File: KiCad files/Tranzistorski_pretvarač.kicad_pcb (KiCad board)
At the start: 2 copper layers, 99.9 x 92.6 mm, 30 parts, among them J1 Screw_Terminal_01x01, J2 Screw_Terminal_01x01, J3 Conn_01x03_Male, J4 Conn_01x01_Male, J5 Screw_Terminal_01x01, J6 Conn_01x01_Male, J7 Conn_01x01_Male, J8 Conn_01x01_Male, J9 Screw_Terminal_01x01, Q1 IRLZ44N, U1 SG3524

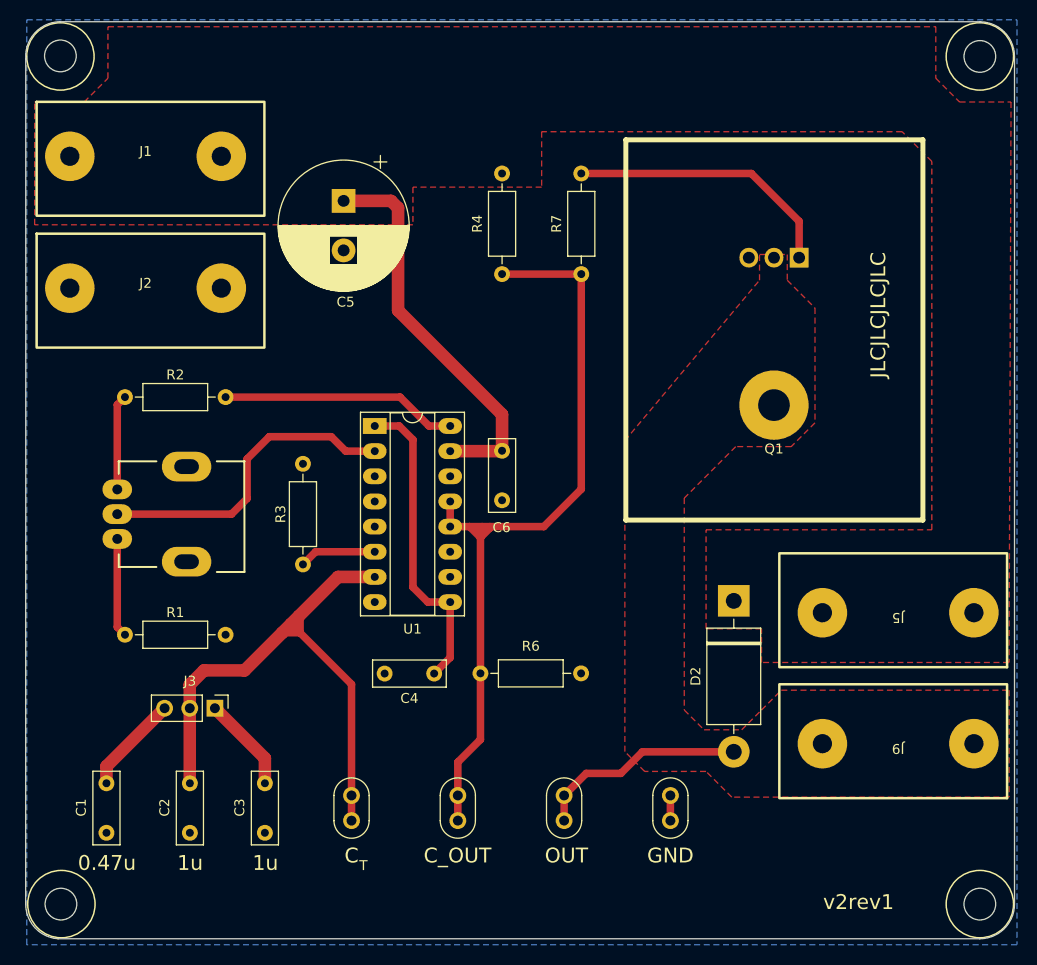
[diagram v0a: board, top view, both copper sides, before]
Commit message: v3
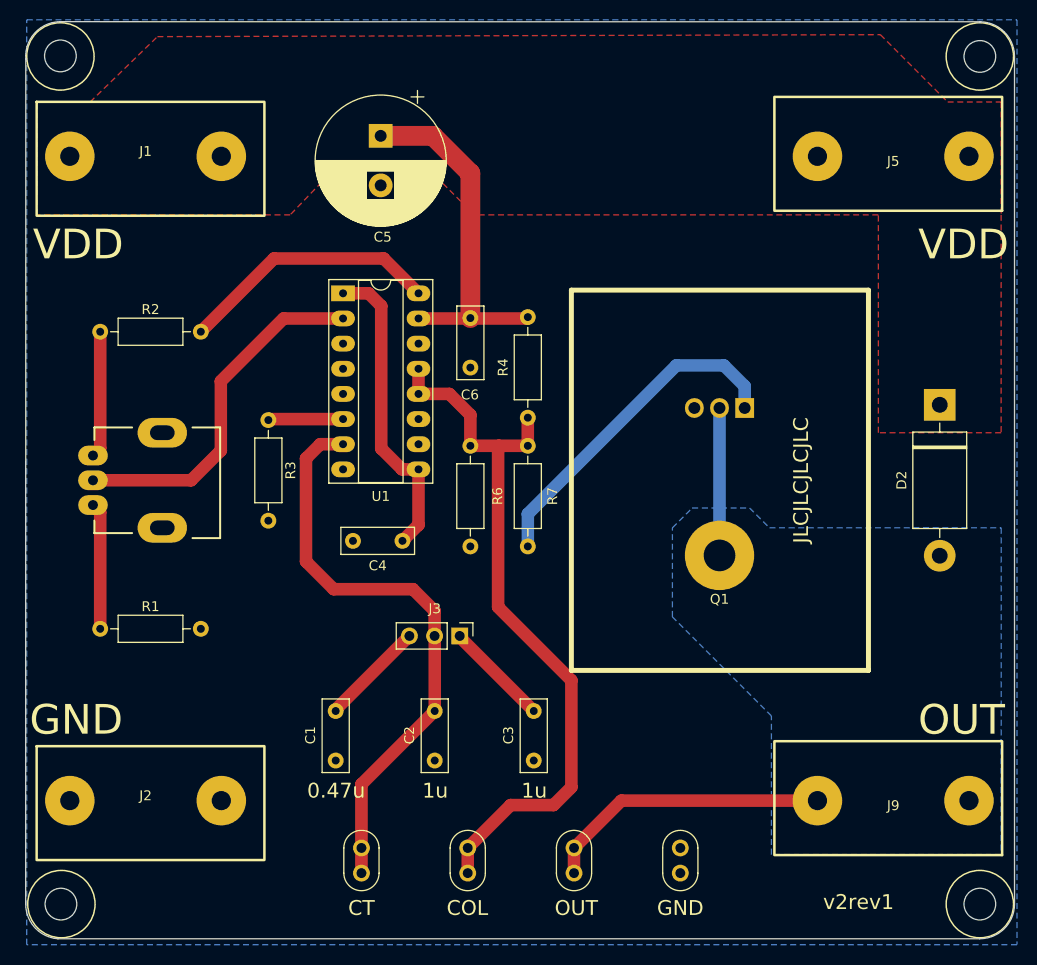
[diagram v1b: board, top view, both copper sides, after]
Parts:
- moved J2 51.8 mm to (101.0, 134.8)
- moved J5 46.1 mm to (176.5, 69.7)
- moved R7 38.0 mm to (139.6, 109.1), turned to 90 degrees
- moved D2 28.7 mm to (181.2, 94.8)
- moved C3 28.1 mm to (140.2, 125.7)
- moved C2 25.8 mm to (130.2, 125.7)
- moved J3 25.8 mm to (132.7, 118.1)
- moved C1 24.3 mm to (120.2, 125.7)
- moved R6 23.0 mm to (133.8, 98.9), turned to -90 degrees
- moved Q1 16.1 mm to (161.5, 95.1)
- moved R3 15.0 mm to (113.4, 96.3), turned to -90 degrees
- moved R4 14.7 mm to (139.6, 85.9)
- moved C4 13.8 mm to (126.9, 108.5)
- moved U1 13.8 mm to (120.9, 83.5)
- moved C6 13.8 mm to (133.8, 86.0)
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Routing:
- net Net-(D2-Pad2): track 21.5 -> 44.0 mm
- net Net-(J6-Pad1): track 80.8 -> 73.5 mm
- net Net-(Q1-Pad1): track 27.7 -> 34.5 mm
- net Net-(RV1-Pad2): track 32.2 -> 36.1 mm
- net VDD: track 39.9 -> 36.3 mm
- net Net-(R2-Pad2): track 9.64 -> 12.8 mm
- net Net-(R1-Pad1): track 10.0 -> 12.8 mm
- net /+5V_REF: track 23.9 -> 26.5 mm
- net GND: track 2.54 -> 0.00 mm
- net Net-(C3-Pad1): track 9.67 -> 10.7 mm
- net Net-(C1-Pad1): track 10.0 -> 10.7 mm
- added copper zone on B.Cu, net Net-(D2-Pad2)
- removed copper zone on F.Cu, net Net-(D2-Pad2)
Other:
- board text added: "COL"
- board text added: "CT"
- board text added: "VDD"
- board text removed: "C"
- board text removed: "C_OUT"
- board text removed: "T"
